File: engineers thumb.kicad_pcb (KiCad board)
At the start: 2 copper layers, 68.6 x 91.4 mm, 55 parts, among them J1 Conn_01x01, J10 Conn_01x01, J11 Conn_01x01, J12 Conn_01x01, J2 Conn_01x01, J3 Conn_01x01, J4 Conn_01x01, J5 Conn_01x01, J6 Conn_01x01, J7 Conn_01x01, J8 Conn_01x01, J9 Conn_01x01, Q1 Q_PMOS_GSD, Q2 BC327, U1 TL072, U2 TL072, U3 LM13700

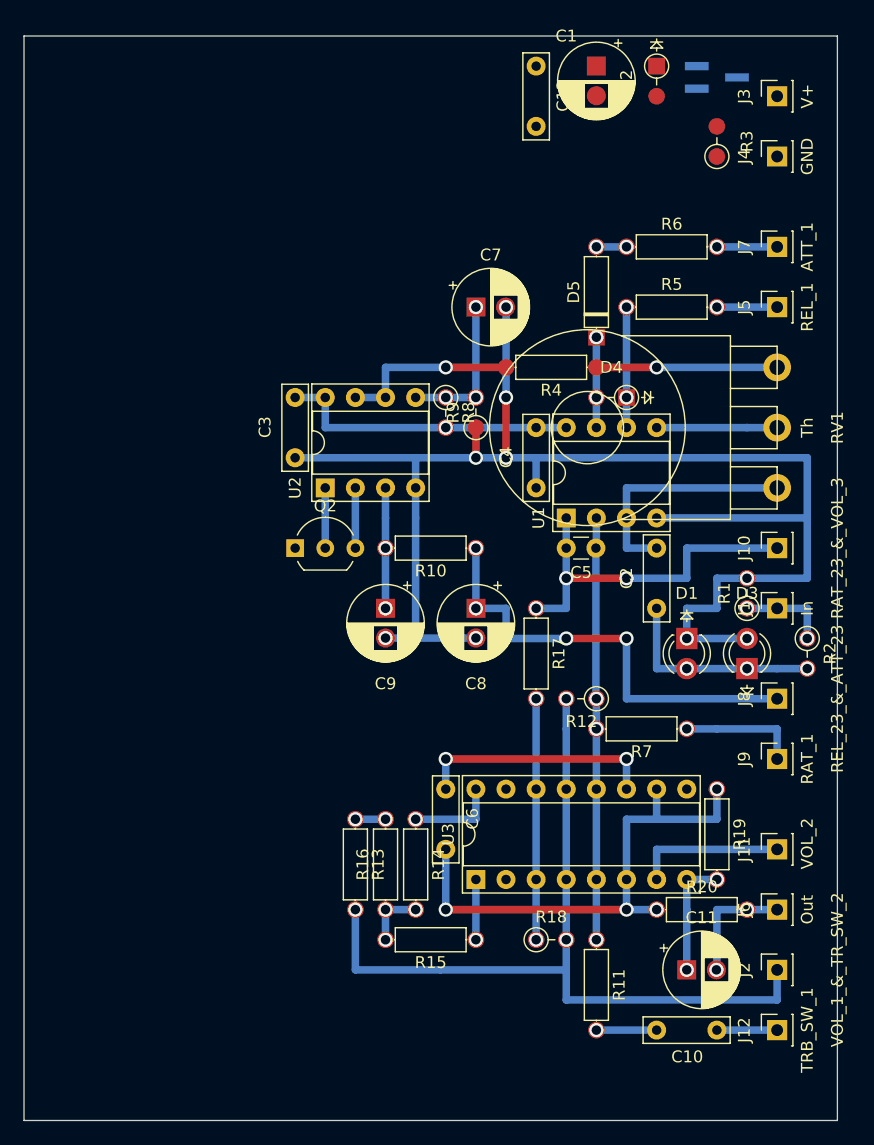
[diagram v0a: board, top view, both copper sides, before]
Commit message: Finnished?
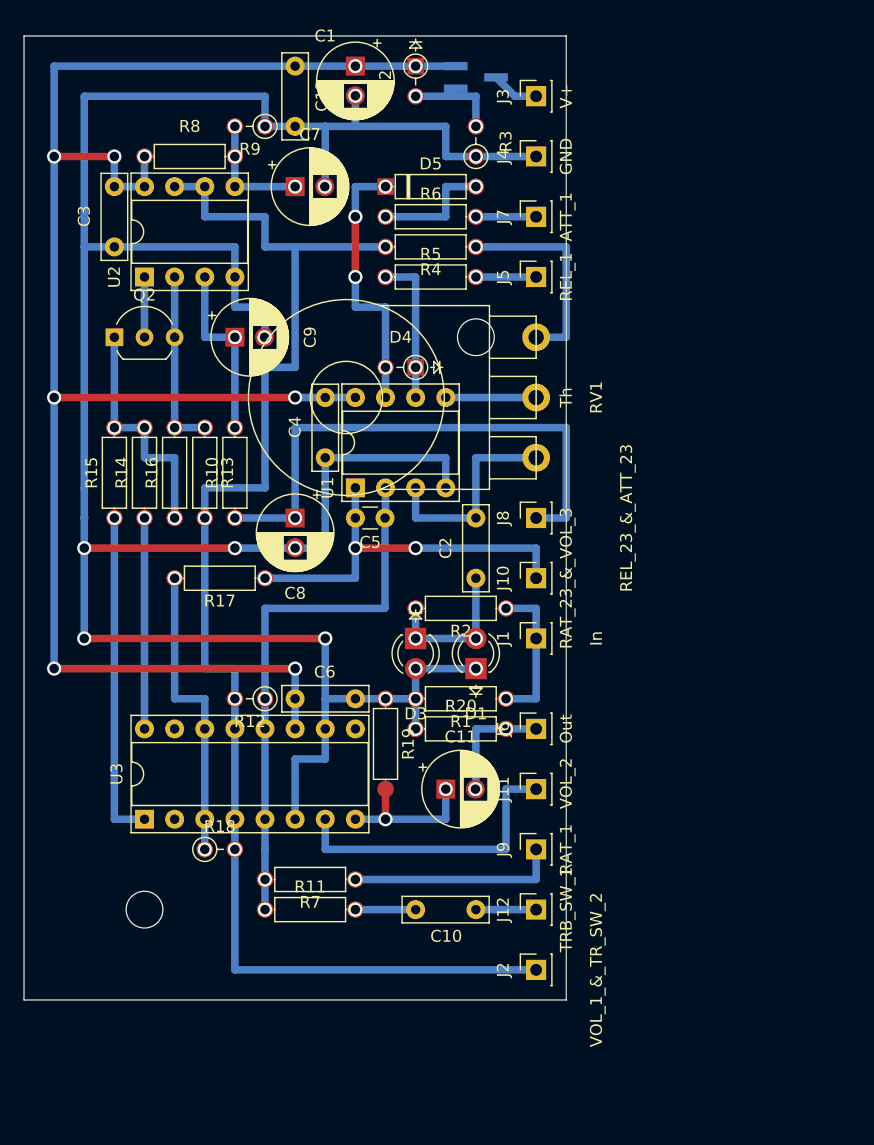
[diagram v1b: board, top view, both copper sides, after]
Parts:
- R1, R2, R8: footprint 2.Breadboard components:R_Axial_Vertical -> 2.Breadboard components:R_Axial_Horizontal
- moved R15 46.8 mm to (43.2, 66.0), turned to 90 degrees
- moved R16 37.5 mm to (48.3, 66.0)
- moved R13 35.4 mm to (50.8, 58.4)
- moved R14 34.2 mm to (45.7, 66.0), turned to 90 degrees
- moved R9 31.0 mm to (55.9, 33.0), turned to 180 degrees
- moved R7 30.7 mm to (63.5, 96.5)
- moved R19 29.0 mm to (66.0, 81.3)
- moved R18 29.0 mm to (50.8, 94.0)
- moved U3 28.4 mm to (45.7, 91.4)
- moved D3 28.1 mm to (68.6, 76.2), turned to 270 degrees
- moved R11 28.1 mm to (55.9, 99.1), turned to 0 degrees
- moved R12 27.9 mm to (55.9, 81.3)
- moved R8 27.0 mm to (53.3, 35.6), turned to 180 degrees
- moved C9 26.2 mm to (53.3, 50.8), turned to 0 degrees
- moved R2 25.5 mm to (76.2, 73.7), turned to 180 degrees
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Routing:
- net +9V: track 45.7 -> 148.2 mm, vias 3 -> 9
- net GND: track 170.2 -> 216.0 mm, vias 13 -> 15
- net +4V5: track 83.8 -> 119.4 mm
- net Net-(R15-Pad1): track 5.08 -> 27.9 mm
- net Net-(Q2-Pad1): track 5.08 -> 20.3 mm
- net Net-(D4-Pad2): track 7.62 -> 22.9 mm, vias 2 -> 4
- net Net-(J11-Pad1): track 12.7 -> 25.4 mm
- net Net-(R14-Pad1): track 7.62 -> 17.8 mm
- net Net-(C5-Pad1): track 35.6 -> 45.7 mm
- net Net-(D2-Pad2): track 0.00 -> 8.73 mm, vias 0 -> 2
- net Net-(C8-Pad1): track 38.1 -> 45.7 mm, vias 4 -> 2
- net Net-(Q2-Pad3): track 7.62 -> 15.2 mm
- net Net-(D5-Pad2): track 2.54 -> 10.2 mm
- net Net-(J9-Pad1): track 10.2 -> 17.8 mm
- net Net-(C9-Pad1): track 10.2 -> 15.2 mm
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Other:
- board size 68.6 x 91.4 mm -> 45.7 x 81.3 mm
